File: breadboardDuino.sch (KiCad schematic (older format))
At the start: 15 parts, among them J3 D-OUT, J4 A-OUT, J5 P-OUT, SW1 SPST, U1 ATMEGA328-PU, X1 16MHZ

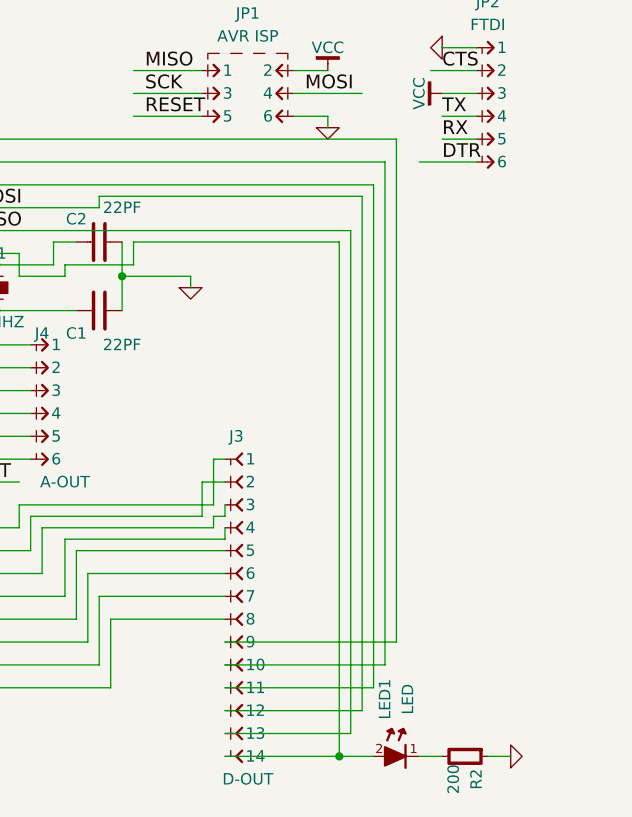
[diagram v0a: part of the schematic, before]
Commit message: Inital layout
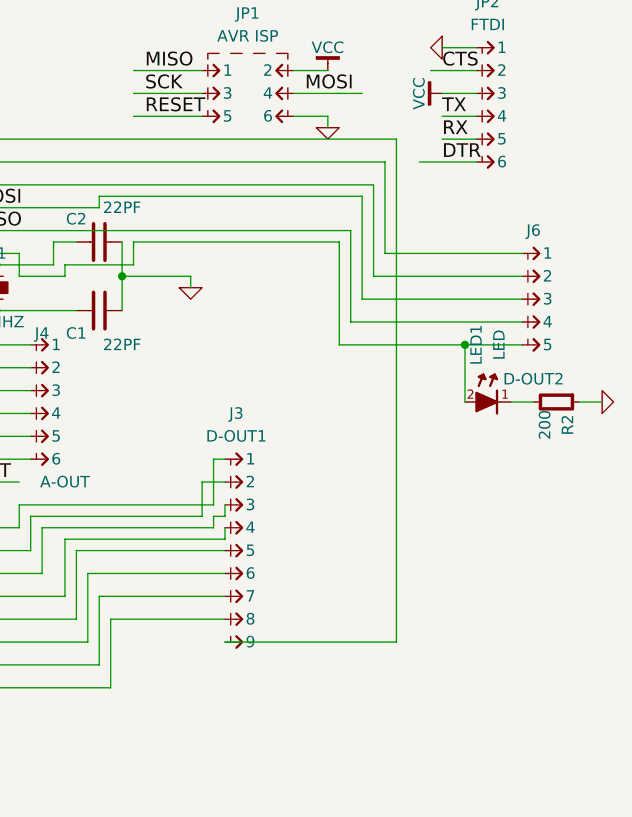
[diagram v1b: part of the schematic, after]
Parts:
- removed J3: D-OUT, conn-100mil:CONN-100MIL-F-1x14, symbol CONN-100MIL-F-1x14
- added J3: D-OUT1, conn-100mil:CONN-100MIL-M-1x9, symbol CONN-100MIL-M-1x9
- added J6: D-OUT2, conn-100mil:CONN-100MIL-M-1x5, symbol CONN-100MIL-M-1x5
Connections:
- wire segments 117 -> 118
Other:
- moved on the sheet: LED1, R2
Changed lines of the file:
@@
 LIBS:Winbond
 LIBS:Xilinx
+LIBS:breadboardDuino-cache
 EELAYER 25 0
 EELAYER END
@@
 DTR
 $Comp
-L CONN-100MIL-F-1x14 J3
-U 1 1 58F7E90F
-P 7900 2850
-F 0 "J3" H 7900 2950 50  0000 C CNN
-F 1 "D-OUT" H 7950 1450 50  0000 C CNN
-F 2 "conn-100mil:CONN-100MIL-F-1x14" H 7900 2850 50  0001 C CNN
-F 3 "" H 7900 2850 50  0000 C CNN
-	1    7900 2850
-	1    0    0    -1
-$EndComp
-$Comp
 L LED LED1
 U 1 1 58F7EBC8
-P 8600 4150
-F 0 "LED1" H 8850 4200 50  0000 C CNN
-F 1 "LED" H 8850 4100 50  0000 C CNN
-F 2 "pth-semi:LED-5mm" H 8600 4150 60  0001 C CNN
-F 3 "" H 8600 4150 60  0000 C CNN
-	1    8600 4150
+P 9000 2600
+F 0 "LED1" H 9250 2650 50  0000 C CNN
+F 1 "LED" H 9250 2550 50  0000 C CNN
+F 2 "pth-semi:LED-5mm" H 9000 2600 60  0001 C CNN
+F 3 "" H 9000 2600 60  0000 C CNN
+	1    9000 2600
 	0    -1   -1   0
 $EndComp
@@
 L R R2
 U 1 1 58F7ECFA
-P 8900 4150
-F 0 "R2" H 9000 4200 50  0000 C CNN
-F 1 "200" H 9000 4100 50  0000 C CNN
-F 2 "pth-passive:R-125mW" H 8900 4200 60  0001 C CNN
-F 3 "" H 8900 4200 60  0000 C CNN
-	1    8900 4150
+P 9300 2600
+F 0 "R2" H 9400 2650 50  0000 C CNN
+F 1 "200" H 9400 2550 50  0000 C CNN
+F 2 "pth-passive:R-125mW" H 9300 2650 60  0001 C CNN
+F 3 "" H 9300 2650 60  0000 C CNN
+	1    9300 2600
 	0    1    1    0
 $EndComp
@@
 L GND #PWR08
 U 1 1 58F7EDEF
-P 9100 4150
-F 0 "#PWR08" H 9100 4150 30  0001 C CNN
-F 1 "GND" H 9100 4080 30  0001 C CNN
-F 2 "" H 9100 4150 60  0000 C CNN
-F 3 "" H 9100 4150 60  0000 C CNN
-	1    9100 4150
+P 9500 2600
+F 0 "#PWR08" H 9500 2600 30  0001 C CNN
+F 1 "GND" H 9500 2530 30  0001 C CNN
+F 2 "" H 9500 2600 60  0000 C CNN
+F 3 "" H 9500 2600 60  0000 C CNN
+	1    9500 2600
 	0    -1   -1   0
 $EndComp
@@
 	4400 2850 4400 3000
 Wire Wire Line
-	8700 4150 8800 4150
-Wire Wire Line
-	9000 4150 9100 4150
+	9100 2600 9200 2600
+Wire Wire Line
+	9400 2600 9500 2600
 Wire Wire Line
 	8950 1350 8800 1350
@@
 	8600 3650 7850 3650
 Wire Wire Line
-	7850 3750 8550 3750
-Wire Wire Line
-	8550 3750 8550 1550
-Wire Wire Line
 	8550 1550 6600 1550
 Wire Wire Line
 	6600 1650 8500 1650
 Wire Wire Line
-	8500 1650 8500 3850
-Wire Wire Line
-	8500 3850 7850 3850
-Wire Wire Line
 	7300 1750 7300 1700
 Wire Wire Line
 	7300 1700 8450 1700
 Wire Wire Line
-	8450 1700 8450 3950
-Wire Wire Line
-	8450 3950 7850 3950
-Wire Wire Line
-	8400 1850 8400 4050
-Wire Wire Line
-	8400 4050 7850 4050
-Wire Wire Line
-	7850 4150 8500 4150
-Wire Wire Line
-	8350 4150 8350 1900
-Wire Wire Line
 	8350 1900 7450 1900
 Wire Wire Line
@@
 Wire Wire Line
 	6950 2050 6950 1950
-Connection ~ 8350 4150
 $Comp
 L CONN-100MIL-M-1x6 J4
@@
 	0    1    1    0
 $EndComp
+$Comp
+L CONN-100MIL-M-1x5 J6
+U 1 1 58FA6D77
+P 9200 1950
+F 0 "J6" H 9200 2050 50  0000 C CNN
+F 1 "D-OUT2" H 9200 1400 50  0000 C CNN
+F 2 "conn-100mil:CONN-100MIL-M-1x5" H 9200 1950 50  0001 C CNN
+F 3 "" H 9200 1950 50  0000 C CNN
+	1    9200 1950
+	1    0    0    -1
+$EndComp
+Wire Wire Line
+	8550 1550 8550 1950
+Wire Wire Line
+	8550 1950 9150 1950
+Wire Wire Line
+	8500 1650 8500 2050
+Wire Wire Line
+	8500 2050 9150 2050
+Wire Wire Line
+	8450 1700 8450 2150
+Wire Wire Line
+	8450 2150 9150 2150
+Wire Wire Line
+	8400 1850 8400 2250
+Wire Wire Line
+	8400 2250 9150 2250
+Wire Wire Line
+	8350 1900 8350 2350
+Wire Wire Line
+	8350 2350 9150 2350
+Wire Wire Line
+	8900 2350 8900 2600
+Connection ~ 8900 2350
+$Comp
+L CONN-100MIL-M-1x9 J3
+U 1 1 58FA76BC
+P 7900 2850
+F 0 "J3" H 7900 3050 50  0000 C CNN
+F 1 "D-OUT1" H 7900 2950 50  0000 C CNN
+F 2 "conn-100mil:CONN-100MIL-M-1x9" H 7900 2850 50  0001 C CNN
+F 3 "" H 7900 2850 50  0000 C CNN
+	1    7900 2850
+	1    0    0    -1
+$EndComp
 $EndSCHEMATC

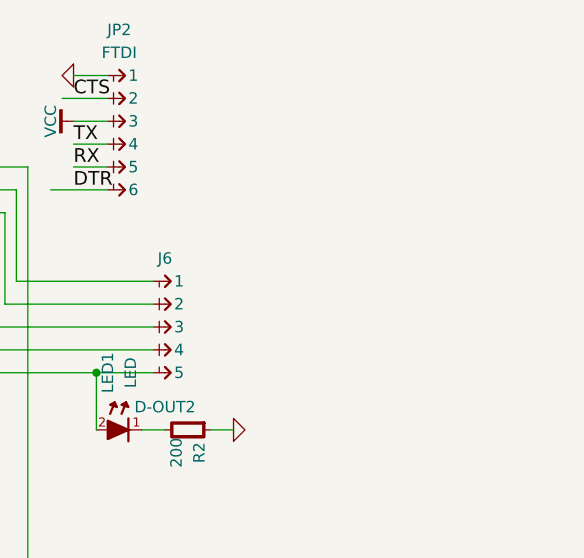
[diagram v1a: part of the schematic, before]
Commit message: Added some proto on the eges
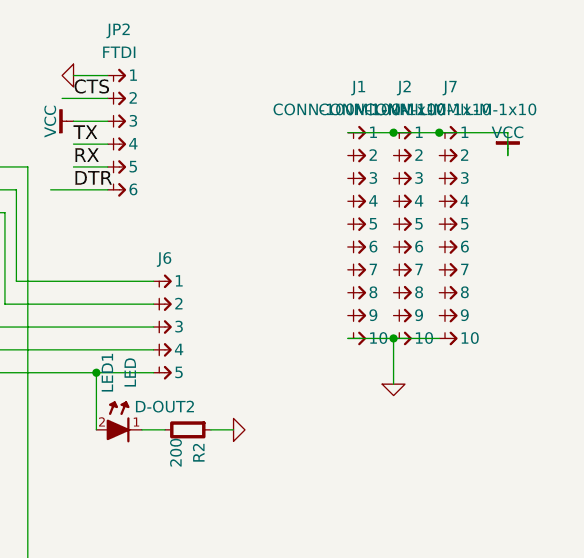
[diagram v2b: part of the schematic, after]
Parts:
- added J1, J2, J7: CONN-100MIL-M-1x10, conn-100mil:CONN-100MIL-M-1x10, symbol CONN-100MIL-M-1x10
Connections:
- wire segments 118 -> 122
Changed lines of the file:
@@
 	1    0    0    -1
 $EndComp
+$Comp
+L CONN-100MIL-M-1x10 J1
+U 1 1 58FA772B
+P 10050 1300
+F 0 "J1" H 10050 1500 50  0000 C CNN
+F 1 "CONN-100MIL-M-1x10" H 10050 1400 50  0000 C CNN
+F 2 "conn-100mil:CONN-100MIL-M-1x10" H 10050 1300 50  0001 C CNN
+F 3 "" H 10050 1300 50  0000 C CNN
+	1    10050 1300
+	1    0    0    -1
+$EndComp
+$Comp
+L CONN-100MIL-M-1x10 J2
+U 1 1 58FA7861
+P 10250 1300
+F 0 "J2" H 10250 1500 50  0000 C CNN
+F 1 "CONN-100MIL-M-1x10" H 10250 1400 50  0000 C CNN
+F 2 "conn-100mil:CONN-100MIL-M-1x10" H 10250 1300 50  0001 C CNN
+F 3 "" H 10250 1300 50  0000 C CNN
+	1    10250 1300
+	1    0    0    -1
+$EndComp
+$Comp
+L CONN-100MIL-M-1x10 J7
+U 1 1 58FA78A6
+P 10450 1300
+F 0 "J7" H 10450 1500 50  0000 C CNN
+F 1 "CONN-100MIL-M-1x10" H 10450 1400 50  0000 C CNN
+F 2 "conn-100mil:CONN-100MIL-M-1x10" H 10450 1300 50  0001 C CNN
+F 3 "" H 10450 1300 50  0000 C CNN
+	1    10450 1300
+	1    0    0    -1
+$EndComp
+Wire Wire Line
+	10000 2200 10400 2200
+Connection ~ 10200 2200
+$Comp
+L VCC #PWR010
+U 1 1 58FA7D17
+P 10700 1400
+F 0 "#PWR010" H 10700 1450 30  0001 C CNN
+F 1 "VCC" H 10700 1500 50  0000 C CNN
+F 2 "" H 10700 1400 60  0000 C CNN
+F 3 "" H 10700 1400 60  0000 C CNN
+	1    10700 1400
+	1    0    0    -1
+$EndComp
+Wire Wire Line
+	10000 1300 10700 1300
+Wire Wire Line
+	10700 1300 10700 1400
+Connection ~ 10200 1300
+Connection ~ 10400 1300
+$Comp
+L GND #PWR?
+U 1 1 58FA8307
+P 10200 2400
+F 0 "#PWR?" H 10200 2400 30  0001 C CNN
+F 1 "GND" H 10200 2330 30  0001 C CNN
+F 2 "" H 10200 2400 60  0000 C CNN
+F 3 "" H 10200 2400 60  0000 C CNN
+	1    10200 2400
+	1    0    0    -1
+$EndComp
+Wire Wire Line
+	10200 2200 10200 2400
 $EndSCHEMATC
